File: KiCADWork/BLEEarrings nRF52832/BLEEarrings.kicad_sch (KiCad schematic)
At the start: 3 parts, among them J3 USB_C_Receptacle, SW1 TK-6580B-1

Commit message: Ignoring Backups
More Dock progress
All local backups removed
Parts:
- J3: LCSC Part (none) -> C5156605
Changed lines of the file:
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@@
+      (effects (font (size 1.27 1.27)) hide)
+    )
+    (property "LCSC Part" "C5156605 " (at 76.835 94.615 0)
       (effects (font (size 1.27 1.27)) hide)
     )

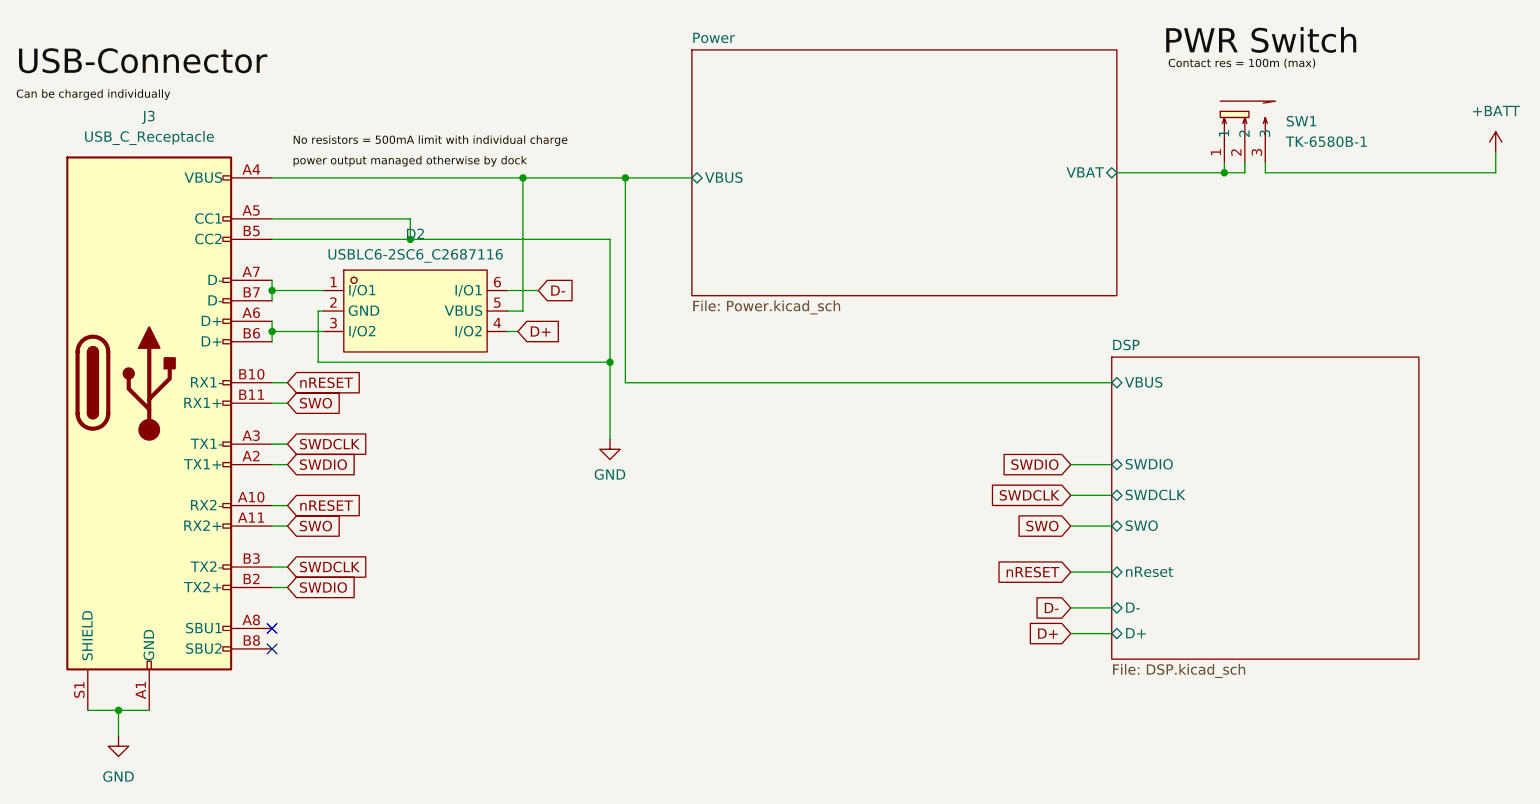
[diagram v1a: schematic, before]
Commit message: Beautiful Skilkscreen Added
Dock schematic intial draft complete
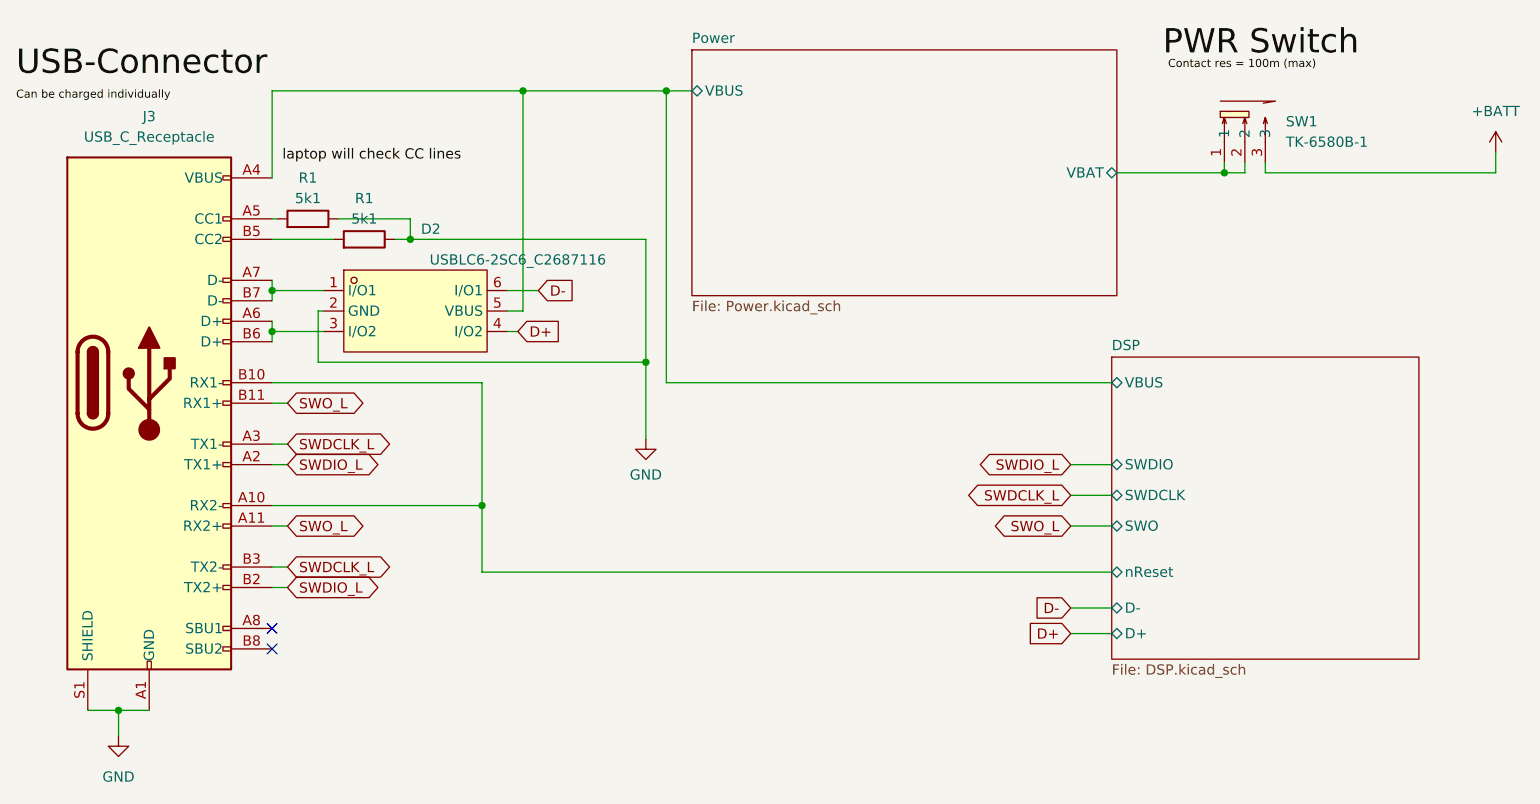
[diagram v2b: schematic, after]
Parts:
- added R1 (x2): 5k1, Resistor_SMD:R_0402_1005Metric_Pad0.72x0.64mm_HandSolder, symbol Device:R
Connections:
- net GND: now also R1.1, R1.1; no longer J3.A5 (CC1), J3.B5 (CC2)
- net SWDCLK renamed SWDCLK_L
- net SWDIO renamed SWDIO_L
- net SWO renamed SWO_L
- net nRESET renamed DSP/nReset
- new net: J3.A5 (CC1), R1.2
- new net: J3.B5 (CC2), R1.2
